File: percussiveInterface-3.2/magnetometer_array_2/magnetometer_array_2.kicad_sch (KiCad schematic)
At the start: 52 parts, among them J1 Conn_01x05_Socket, J2 Conn_01x12_Socket, J3 Conn_01x12_Socket, J4 Conn_01x12_Socket, U1 SM225-10E, U10 SM225-10E, U11 SM225-10E, U12 SM225-10E, U13 SM225-10E, U14 SM225-10E, U15 SM225-10E, U16 SM225-10E, U17 SM225-10E, U18 SM225-10E, U19 SM225-10E, U2 SM225-10E, U20 SM225-10E, U21 SM225-10E, U22 SM225-10E, U23 SM225-10E, U24 SM225-10E, U3 SM225-10E, U4 SM225-10E, U5 SM225-10E, U6 SM225-10E, U7 SM225-10E, U8 SM225-10E, U9 SM225-10E

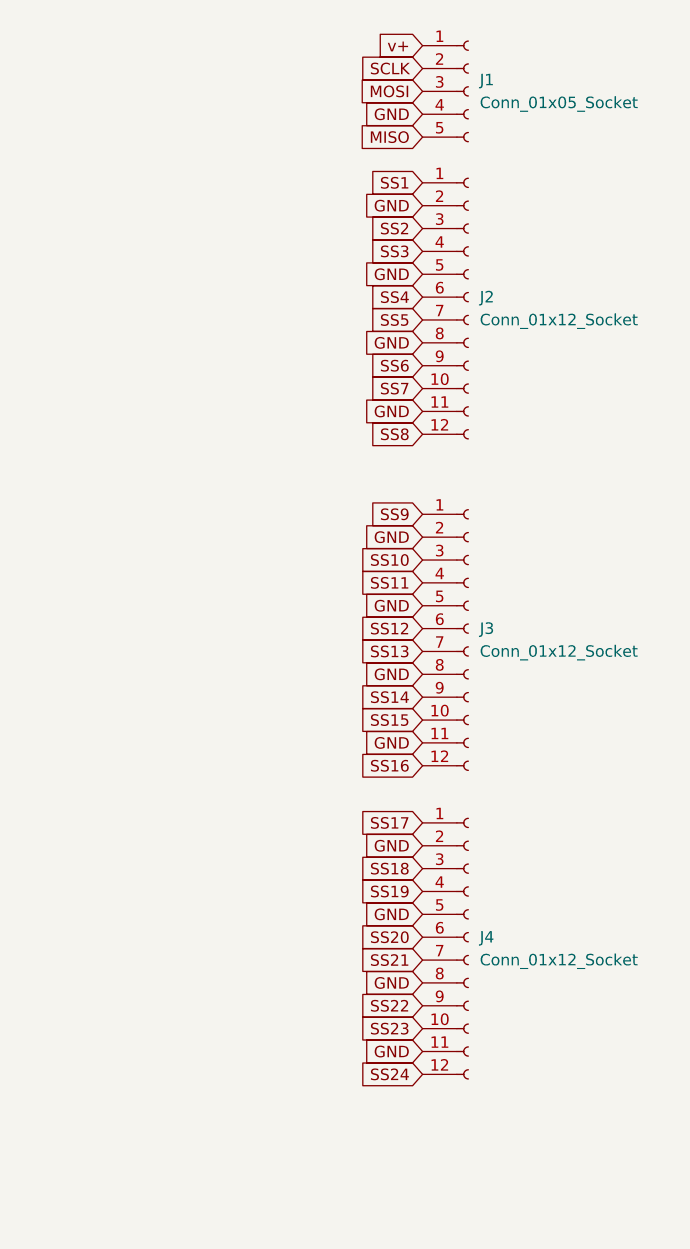
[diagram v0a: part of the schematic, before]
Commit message: many changes
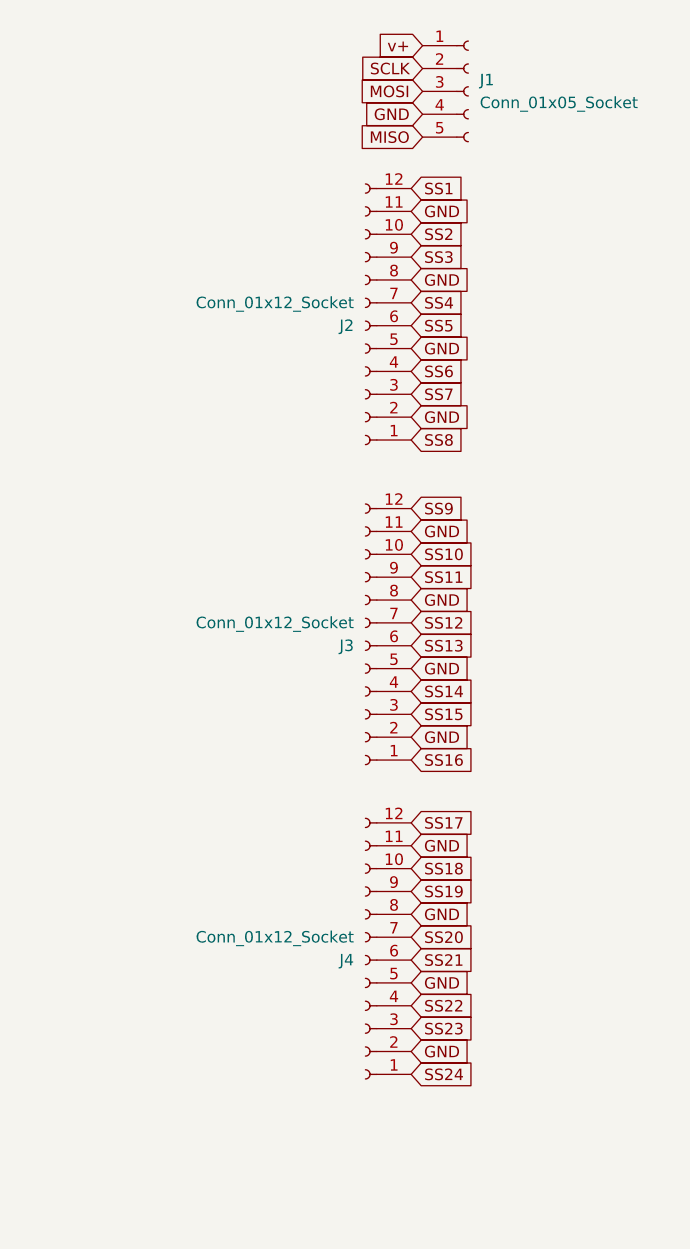
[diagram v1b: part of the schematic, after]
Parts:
- J1: footprint Connector_Harwin:Harwin_M20-89005xx_1x05_P2.54mm_Horizontal -> Connector_PinHeader_2.54mm:PinHeader_1x05_P2.54mm_Horizontal
- J2, J3, J4: footprint Connector_Harwin:Harwin_M20-89012xx_1x12_P2.54mm_Horizontal -> Connector_PinHeader_2.54mm:PinHeader_1x12_P2.54mm_Horizontal
- U1, U10, U11, U12, U13, U14, U15, U16, U17, U18, U19, U2, U20, U21, U22, U23, U24, U3, U4, U5, U6, U7, U8, U9: footprint own_footprints:NVE SM225 10E -> Own_Library:NVE SM225 10E
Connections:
- net SS1: now also J2.12 (Pin_12); no longer J2.1 (Pin_1)
- net SS10: now also J3.10 (Pin_10); no longer J3.3 (Pin_3)
- net SS11: now also J3.9 (Pin_9); no longer J3.4 (Pin_4)
- net SS12: now also J3.7 (Pin_7); no longer J3.6 (Pin_6)
- net SS13: now also J3.6 (Pin_6); no longer J3.7 (Pin_7)
- net SS14: now also J3.4 (Pin_4); no longer J3.9 (Pin_9)
- net SS15: now also J3.3 (Pin_3); no longer J3.10 (Pin_10)
- net SS16: now also J3.1 (Pin_1); no longer J3.12 (Pin_12)
- net SS17: now also J4.12 (Pin_12); no longer J4.1 (Pin_1)
- net SS18: now also J4.10 (Pin_10); no longer J4.3 (Pin_3)
- net SS19: now also J4.9 (Pin_9); no longer J4.4 (Pin_4)
- net SS2: now also J2.10 (Pin_10); no longer J2.3 (Pin_3)
- net SS20: now also J4.7 (Pin_7); no longer J4.6 (Pin_6)
- net SS21: now also J4.6 (Pin_6); no longer J4.7 (Pin_7)
- net SS22: now also J4.4 (Pin_4); no longer J4.9 (Pin_9)
- net SS23: now also J4.3 (Pin_3); no longer J4.10 (Pin_10)
- net SS24: now also J4.1 (Pin_1); no longer J4.12 (Pin_12)
- net SS3: now also J2.9 (Pin_9); no longer J2.4 (Pin_4)
- net SS4: now also J2.7 (Pin_7); no longer J2.6 (Pin_6)
- net SS5: now also J2.6 (Pin_6); no longer J2.7 (Pin_7)
- net SS6: now also J2.4 (Pin_4); no longer J2.9 (Pin_9)
- net SS7: now also J2.3 (Pin_3); no longer J2.10 (Pin_10)
- net SS8: now also J2.1 (Pin_1); no longer J2.12 (Pin_12)
- net SS9: now also J3.12 (Pin_12); no longer J3.1 (Pin_1)
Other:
- moved on the sheet: J2, J3, J4
